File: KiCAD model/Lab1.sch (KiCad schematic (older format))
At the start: 116 parts, among them J1 USB_OTG, J2 SWD, SW1 Reset, SW10 Rotary_Encoder, SW2 Reset, SW3 Reset, SW4 Reset, SW5 Reset, SW6 Reset, SW7 Reset, SW9 Reset, U1 PMW3389, U2 AP2125N-3.3TRG, U3 MIC5235YM5-TR, U4 STM32F411RETx, U5 USBLC6-2SC6, Y1 16Mhz

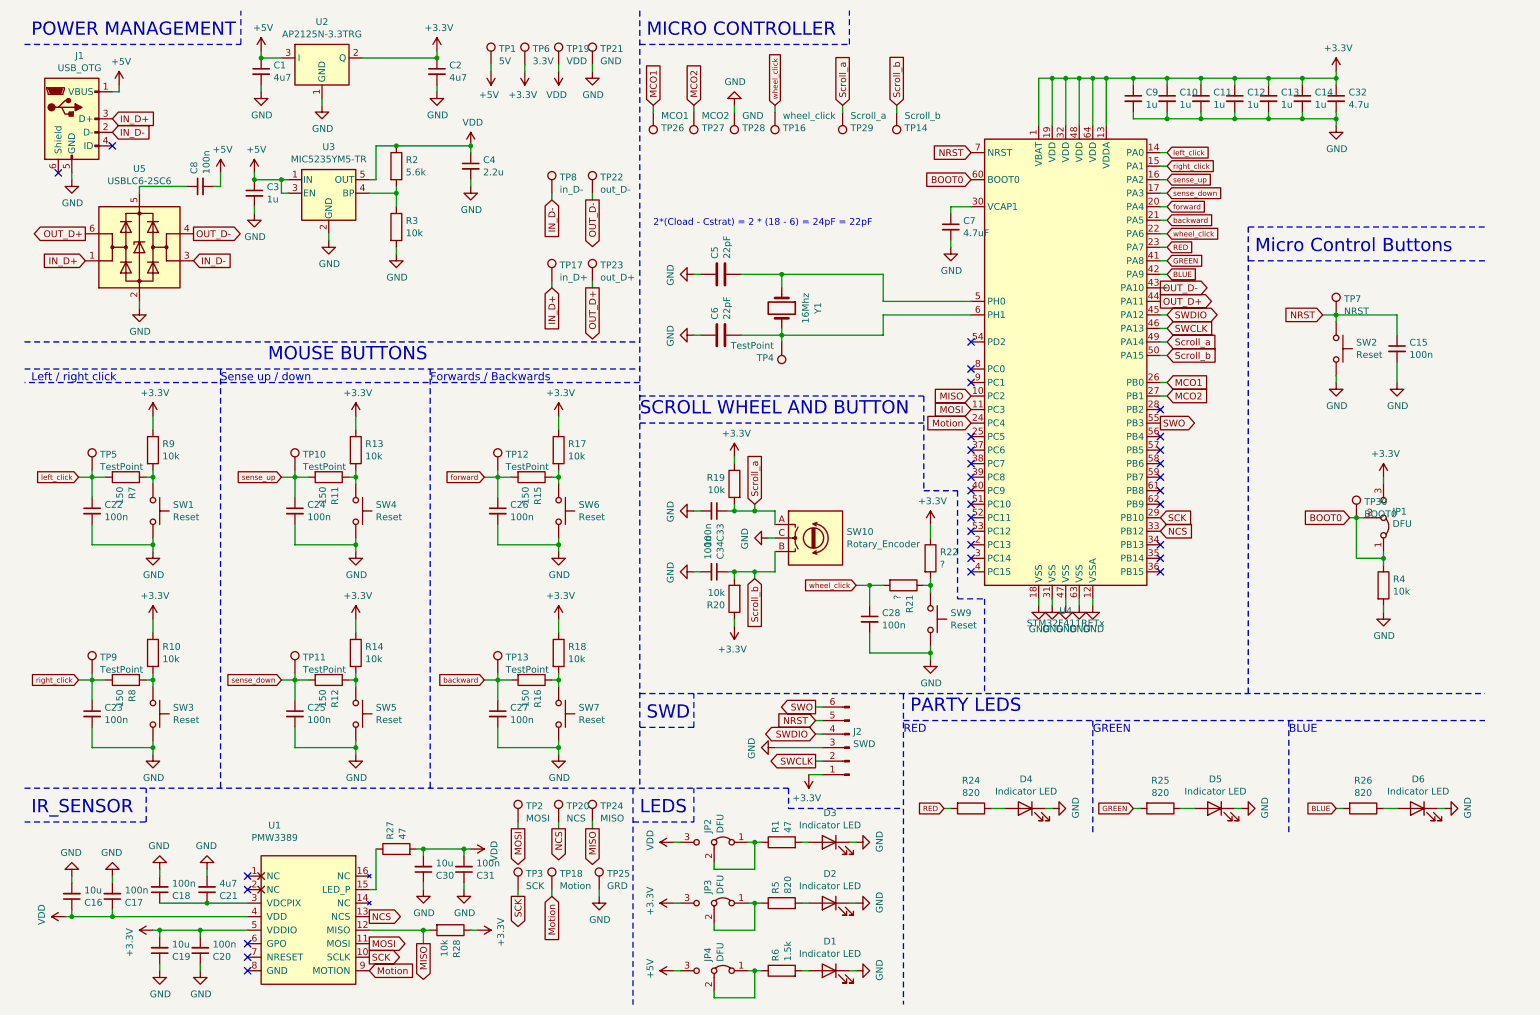
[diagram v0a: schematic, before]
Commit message: orgot the model
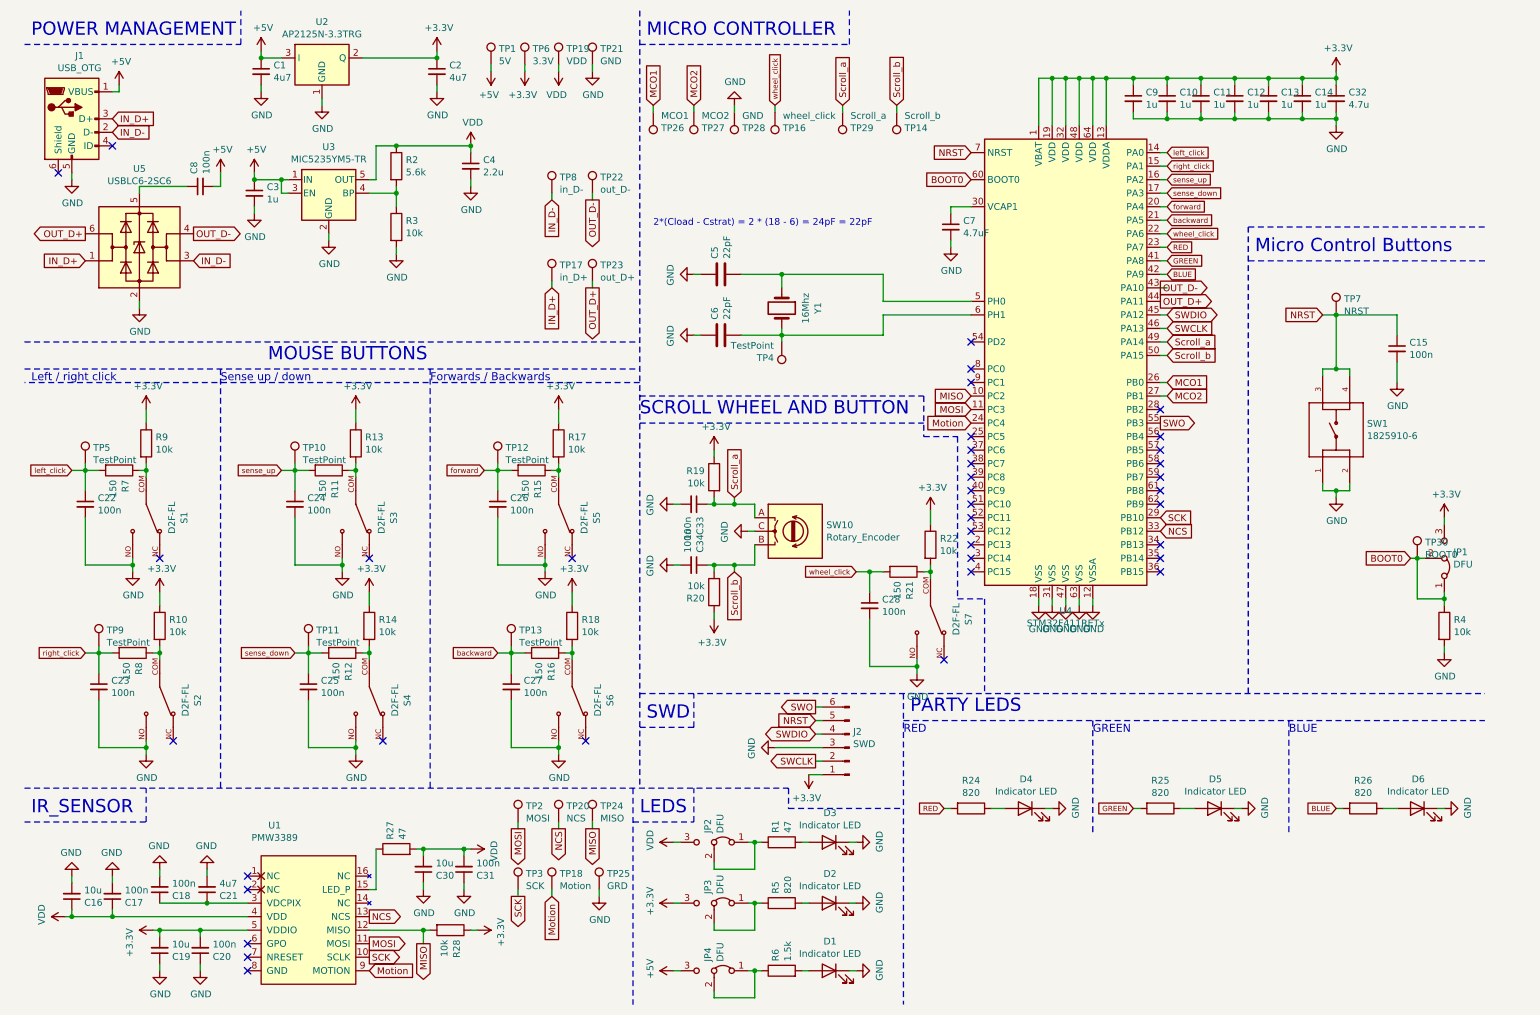
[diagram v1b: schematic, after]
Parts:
- removed SW1, SW2, SW3, SW4, SW5, SW6, SW7, SW9: Reset, Button_Switch_SMD:SW_SPST_B3U-1000P, symbol Switch:SW_Push
- added S1, S2, S3, S4, S5, S6, S7: D2F-FL, Desktop:SW_D2F-FL, symbol D2F-FL:D2F-FL
- added SW1: 1825910-6, Desktop:SW_1825910-6-4, symbol 1825910-6:1825910-6
- R21: value ? -> 150
- R22: value ? -> 10k
- U1: footprint Battery:PMW3389 -> Custom:PMW3389
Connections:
- net GND: now also S1.NO, S2.NO, S3.NO, S4.NO, S5.NO, S6.NO, S7.NO, SW1.1, SW1.2
- net NRST: now also SW1.3, SW1.4
- net at R12.1, R14.2: now also S4.COM
- net at R11.1, R13.2: now also S3.COM
- net at R16.1, R18.2: now also S6.COM
- net at R15.1, R17.2: now also S5.COM
- net at R10.2, R8.1: now also S2.COM
- net at R7.1, R9.2: now also S1.COM
- net at R21.1, R22.2: now also S7.COM
- no-connect marks 31 -> 38
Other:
- moved on the sheet: C22, C28, C33, C34, JP1, R19, R20, R21, R22, R4, R7, R9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

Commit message: Fixed footprint for testpoints
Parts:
- S1, S2, S3, S4, S5, S6, S7: symbol D2F-FL:D2F-FL -> Lab1-rescue:D2F-FL-D2F-FL
- SW1: symbol 1825910-6:1825910-6 -> Lab1-rescue:1825910-6-1825910-6
- TP1, TP10, TP11, TP12, TP13, TP14, TP16, TP17, TP18, TP19, TP2, TP20, TP21, TP22, TP23, TP24, TP25, TP26, TP27, TP28, TP29, TP3, TP30, TP4, TP5, TP6, TP7, TP8, TP9: footprint TestPoint:TestPoint_Pad_1.5x1.5mm -> TestPoint:TestPoint_Keystone_5015_Micro-Minature
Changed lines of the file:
@@
 F 0 "TP7" H 10208 2818 50  0000 L CNN
 F 1 "NRST" H 10208 2727 50  0000 L CNN
-F 2 "TestPoint:TestPoint_Pad_1.5x1.5mm" H 10350 2700 50  0001 C CNN
+F 2 "TestPoint:TestPoint_Keystone_5015_Micro-Minature" H 10350 2700 50  0001 C CNN
 F 3 "~" H 10350 2700 50  0001 C CNN
 	1    10150 2700
@@
 F 0 "TP16" H 6058 1318 50  0000 L CNN
 F 1 "wheel_click" H 6058 1227 50  0000 L CNN
-F 2 "TestPoint:TestPoint_Pad_1.5x1.5mm" H 6200 1200 50  0001 C CNN
+F 2 "TestPoint:TestPoint_Keystone_5015_Micro-Minature" H 6200 1200 50  0001 C CNN
 F 3 "~" H 6200 1200 50  0001 C CNN
 	1    6000 1200
@@
 F 0 "TP20" H 4458 6568 50  0000 L CNN
 F 1 "NCS" H 4458 6477 50  0000 L CNN
-F 2 "TestPoint:TestPoint_Pad_1.5x1.5mm" H 4600 6450 50  0001 C CNN
+F 2 "TestPoint:TestPoint_Keystone_5015_Micro-Minature" H 4600 6450 50  0001 C CNN
 F 3 "~" H 4600 6450 50  0001 C CNN
 	1    4400 6450
@@
 F 0 "TP2" H 4158 6568 50  0000 L CNN
 F 1 "MOSI" H 4158 6477 50  0000 L CNN
-F 2 "TestPoint:TestPoint_Pad_1.5x1.5mm" H 4300 6450 50  0001 C CNN
+F 2 "TestPoint:TestPoint_Keystone_5015_Micro-Minature" H 4300 6450 50  0001 C CNN
 F 3 "~" H 4300 6450 50  0001 C CNN
 	1    4100 6450
@@
 F 0 "TP3" H 4158 7068 50  0000 L CNN
 F 1 "SCK" H 4158 6977 50  0000 L CNN
-F 2 "TestPoint:TestPoint_Pad_1.5x1.5mm" H 4300 6950 50  0001 C CNN
+F 2 "TestPoint:TestPoint_Keystone_5015_Micro-Minature" H 4300 6950 50  0001 C CNN
 F 3 "~" H 4300 6950 50  0001 C CNN
 	1    4100 6950
@@
 F 0 "TP18" H 4408 7068 50  0000 L CNN
 F 1 "Motion" H 4408 6977 50  0000 L CNN
-F 2 "TestPoint:TestPoint_Pad_1.5x1.5mm" H 4550 6950 50  0001 C CNN
+F 2 "TestPoint:TestPoint_Keystone_5015_Micro-Minature" H 4550 6950 50  0001 C CNN
 F 3 "~" H 4550 6950 50  0001 C CNN
 	1    4350 6950
@@
 F 0 "TP24" H 4708 6568 50  0000 L CNN
 F 1 "MISO" H 4708 6477 50  0000 L CNN
-F 2 "TestPoint:TestPoint_Pad_1.5x1.5mm" H 4850 6450 50  0001 C CNN
+F 2 "TestPoint:TestPoint_Keystone_5015_Micro-Minature" H 4850 6450 50  0001 C CNN
 F 3 "~" H 4850 6450 50  0001 C CNN
 	1    4650 6450
@@
 F 0 "TP25" H 4758 7068 50  0000 L CNN
 F 1 "GRD" H 4758 6977 50  0000 L CNN
-F 2 "TestPoint:TestPoint_Pad_1.5x1.5mm" H 4900 6950 50  0001 C CNN
+F 2 "TestPoint:TestPoint_Keystone_5015_Micro-Minature" H 4900 6950 50  0001 C CNN
 F 3 "~" H 4900 6950 50  0001 C CNN
 	1    4700 6950
@@
 F 0 "TP1" H 3958 968 50  0000 L CNN
 F 1 "5V" H 3958 877 50  0000 L CNN
-F 2 "TestPoint:TestPoint_Pad_1.5x1.5mm" H 4100 850 50  0001 C CNN
+F 2 "TestPoint:TestPoint_Keystone_5015_Micro-Minature" H 4100 850 50  0001 C CNN
 F 3 "~" H 4100 850 50  0001 C CNN
 	1    3900 850
@@
 F 0 "TP6" H 4208 968 50  0000 L CNN
 F 1 "3.3V" H 4208 877 50  0000 L CNN
-F 2 "TestPoint:TestPoint_Pad_1.5x1.5mm" H 4350 850 50  0001 C CNN
+F 2 "TestPoint:TestPoint_Keystone_5015_Micro-Minature" H 4350 850 50  0001 C CNN
 F 3 "~" H 4350 850 50  0001 C CNN
 	1    4150 850
@@
 F 0 "TP19" H 4458 968 50  0000 L CNN
 F 1 "VDD" H 4458 877 50  0000 L CNN
-F 2 "TestPoint:TestPoint_Pad_1.5x1.5mm" H 4600 850 50  0001 C CNN
+F 2 "TestPoint:TestPoint_Keystone_5015_Micro-Minature" H 4600 850 50  0001 C CNN
 F 3 "~" H 4600 850 50  0001 C CNN
 	1    4400 850
@@
 F 0 "TP21" H 4708 968 50  0000 L CNN
 F 1 "GND" H 4708 877 50  0000 L CNN
-F 2 "TestPoint:TestPoint_Pad_1.5x1.5mm" H 4850 850 50  0001 C CNN
+F 2 "TestPoint:TestPoint_Keystone_5015_Micro-Minature" H 4850 850 50  0001 C CNN
 F 3 "~" H 4850 850 50  0001 C CNN
 	1    4650 850
@@
 F 0 "TP27" H 5458 1318 50  0000 L CNN
 F 1 "MCO2" H 5458 1227 50  0000 L CNN
-F 2 "TestPoint:TestPoint_Pad_1.5x1.5mm" H 5600 1200 50  0001 C CNN
+F 2 "TestPoint:TestPoint_Keystone_5015_Micro-Minature" H 5600 1200 50  0001 C CNN
 F 3 "~" H 5600 1200 50  0001 C CNN
 	1    5400 1200
@@
 F 0 "TP26" H 5158 1318 50  0000 L CNN
 F 1 "MCO1" H 5158 1227 50  0000 L CNN
-F 2 "TestPoint:TestPoint_Pad_1.5x1.5mm" H 5300 1200 50  0001 C CNN
+F 2 "TestPoint:TestPoint_Keystone_5015_Micro-Minature" H 5300 1200 50  0001 C CNN
 F 3 "~" H 5300 1200 50  0001 C CNN
 	1    5100 1200
@@
 F 0 "TP28" H 5758 1318 50  0000 L CNN
 F 1 "GND" H 5758 1227 50  0000 L CNN
-F 2 "TestPoint:TestPoint_Pad_1.5x1.5mm" H 5900 1200 50  0001 C CNN
+F 2 "TestPoint:TestPoint_Keystone_5015_Micro-Minature" H 5900 1200 50  0001 C CNN
 F 3 "~" H 5900 1200 50  0001 C CNN
 	1    5700 1200
@@
 F 0 "TP29" H 6558 1318 50  0000 L CNN
 F 1 "Scroll_a" H 6558 1227 50  0000 L CNN
-F 2 "TestPoint:TestPoint_Pad_1.5x1.5mm" H 6700 1200 50  0001 C CNN
+F 2 "TestPoint:TestPoint_Keystone_5015_Micro-Minature" H 6700 1200 50  0001 C CNN
 F 3 "~" H 6700 1200 50  0001 C CNN
 	1    6500 1200
@@
 F 0 "TP30" H 10808 4618 50  0000 L CNN
 F 1 "BOOT0" H 10808 4527 50  0000 L CNN
-F 2 "TestPoint:TestPoint_Pad_1.5x1.5mm" H 10950 4500 50  0001 C CNN
+F 2 "TestPoint:TestPoint_Keystone_5015_Micro-Minature" H 10950 4500 50  0001 C CNN
 F 3 "~" H 10950 4500 50  0001 C CNN
 	1    10750 4500
@@
 F 0 "TP17" H 4408 2568 50  0000 L CNN
 F 1 "in_D+" H 4408 2477 50  0000 L CNN
-F 2 "TestPoint:TestPoint_Pad_1.5x1.5mm" H 4550 2450 50  0001 C CNN
+F 2 "TestPoint:TestPoint_Keystone_5015_Micro-Minature" H 4550 2450 50  0001 C CNN
 F 3 "~" H 4550 2450 50  0001 C CNN
 	1    4350 2450
@@
 F 0 "TP23" H 4708 2568 50  0000 L CNN
 F 1 "out_D+" H 4708 2477 50  0000 L CNN
-F 2 "TestPoint:TestPoint_Pad_1.5x1.5mm" H 4850 2450 50  0001 C CNN
+F 2 "TestPoint:TestPoint_Keystone_5015_Micro-Minature" H 4850 2450 50  0001 C CNN
 F 3 "~" H 4850 2450 50  0001 C CNN
 	1    4650 2450
@@
 F 0 "TP8" H 4408 1918 50  0000 L CNN
 F 1 "in_D-" H 4408 1827 50  0000 L CNN
-F 2 "TestPoint:TestPoint_Pad_1.5x1.5mm" H 4550 1800 50  0001 C CNN
+F 2 "TestPoint:TestPoint_Keystone_5015_Micro-Minature" H 4550 1800 50  0001 C CNN
 F 3 "~" H 4550 1800 50  0001 C CNN
 	1    4350 1800
@@
 F 0 "TP22" H 4708 1918 50  0000 L CNN
 F 1 "out_D-" H 4708 1827 50  0000 L CNN
-F 2 "TestPoint:TestPoint_Pad_1.5x1.5mm" H 4850 1800 50  0001 C CNN
+F 2 "TestPoint:TestPoint_Keystone_5015_Micro-Minature" H 4850 1800 50  0001 C CNN
 F 3 "~" H 4850 1800 50  0001 C CNN
 	1    4650 1800
@@
 F 0 "TP14" H 6958 1318 50  0000 L CNN
 F 1 "Scroll_b" H 6958 1227 50  0000 L CNN
-F 2 "TestPoint:TestPoint_Pad_1.5x1.5mm" H 7100 1200 50  0001 C CNN
+F 2 "TestPoint:TestPoint_Keystone_5015_Micro-Minature" H 7100 1200 50  0001 C CNN
 F 3 "~" H 7100 1200 50  0001 C CNN
 	1    6900 1200
@@
 F 0 "TP4" H 6108 3018 50  0000 L CNN
 F 1 "TestPoint" H 6108 2927 50  0000 L CNN
-F 2 "TestPoint:TestPoint_Pad_1.5x1.5mm" H 6250 2900 50  0001 C CNN
+F 2 "TestPoint:TestPoint_Keystone_5015_Micro-Minature" H 6250 2900 50  0001 C CNN
 F 3 "~" H 6250 2900 50  0001 C CNN
 	1    6050 2900
@@
 Scroll_b
 $Comp
-L D2F-FL:D2F-FL S1
+L Lab1-rescue:D2F-FL-D2F-FL S1
 U 1 1 6034E202
 P 1350 4200
@@
 F 0 "TP5" H 958 3918 50  0000 L CNN
 F 1 "TestPoint" H 958 3827 50  0000 L CNN
-F 2 "TestPoint:TestPoint_Pad_1.5x1.5mm" H 1100 3800 50  0001 C CNN
+F 2 "TestPoint:TestPoint_Keystone_5015_Micro-Minature" H 1100 3800 50  0001 C CNN
 F 3 "~" H 1100 3800 50  0001 C CNN
 	1    900  3800
@@
 NoConn ~ 1450 4500
 $Comp
-L D2F-FL:D2F-FL S2
+L Lab1-rescue:D2F-FL-D2F-FL S2
 U 1 1 60880B22
 P 1450 5550
@@
 F 0 "TP9" H 1058 5268 50  0000 L CNN
 F 1 "TestPoint" H 1058 5177 50  0000 L CNN
-F 2 "TestPoint:TestPoint_Pad_1.5x1.5mm" H 1200 5150 50  0001 C CNN
+F 2 "TestPoint:TestPoint_Keystone_5015_Micro-Minature" H 1200 5150 50  0001 C CNN
 F 3 "~" H 1200 5150 50  0001 C CNN
 	1    1000 5150
@@
 NoConn ~ 1550 5850
 $Comp
-L D2F-FL:D2F-FL S3
+L Lab1-rescue:D2F-FL-D2F-FL S3
 U 1 1 608B0D57
 P 2900 4200
@@
 F 0 "TP10" H 2508 3918 50  0000 L CNN
 F 1 "TestPoint" H 2508 3827 50  0000 L CNN
-F 2 "TestPoint:TestPoint_Pad_1.5x1.5mm" H 2650 3800 50  0001 C CNN
+F 2 "TestPoint:TestPoint_Keystone_5015_Micro-Minature" H 2650 3800 50  0001 C CNN
 F 3 "~" H 2650 3800 50  0001 C CNN
 	1    2450 3800
@@
 NoConn ~ 3000 4500
 $Comp
-L D2F-FL:D2F-FL S4
+L Lab1-rescue:D2F-FL-D2F-FL S4
 U 1 1 608E2D04
 P 3000 5550
@@
 F 0 "TP11" H 2608 5268 50  0000 L CNN
 F 1 "TestPoint" H 2608 5177 50  0000 L CNN
-F 2 "TestPoint:TestPoint_Pad_1.5x1.5mm" H 2750 5150 50  0001 C CNN
+F 2 "TestPoint:TestPoint_Keystone_5015_Micro-Minature" H 2750 5150 50  0001 C CNN
 F 3 "~" H 2750 5150 50  0001 C CNN
 	1    2550 5150
@@
 NoConn ~ 3100 5850
 $Comp
-L D2F-FL:D2F-FL S5
+L Lab1-rescue:D2F-FL-D2F-FL S5
 U 1 1 6090304B
 P 4400 4200
@@
 F 0 "TP12" H 4008 3918 50  0000 L CNN
 F 1 "TestPoint" H 4008 3827 50  0000 L CNN
-F 2 "TestPoint:TestPoint_Pad_1.5x1.5mm" H 4150 3800 50  0001 C CNN
+F 2 "TestPoint:TestPoint_Keystone_5015_Micro-Minature" H 4150 3800 50  0001 C CNN
 F 3 "~" H 4150 3800 50  0001 C CNN
 	1    3950 3800
@@
 NoConn ~ 4500 4500
 $Comp
-L D2F-FL:D2F-FL S6
+L Lab1-rescue:D2F-FL-D2F-FL S6
 U 1 1 609243E2
 P 4500 5550
@@
 F 0 "TP13" H 4108 5268 50  0000 L CNN
 F 1 "TestPoint" H 4108 5177 50  0000 L CNN
-F 2 "TestPoint:TestPoint_Pad_1.5x1.5mm" H 4250 5150 50  0001 C CNN
+F 2 "TestPoint:TestPoint_Keystone_5015_Micro-Minature" H 4250 5150 50  0001 C CNN
 F 3 "~" H 4250 5150 50  0001 C CNN
 	1    4050 5150
@@
 $EndComp
 $Comp
-L D2F-FL:D2F-FL S7
+L Lab1-rescue:D2F-FL-D2F-FL S7
 U 1 1 60A1D62C
 P 7150 4950
@@
 	7350 3600 7350 4800
 $Comp
-L 1825910-6:1825910-6 SW1
+L Lab1-rescue:1825910-6-1825910-6 SW1
 U 1 1 60273442
 P 10150 3550
